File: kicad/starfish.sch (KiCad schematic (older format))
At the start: 3 parts, among them J1 Conn_02x04_Counter_Clockwise, J2 Conn_01x04, U1 kmz60

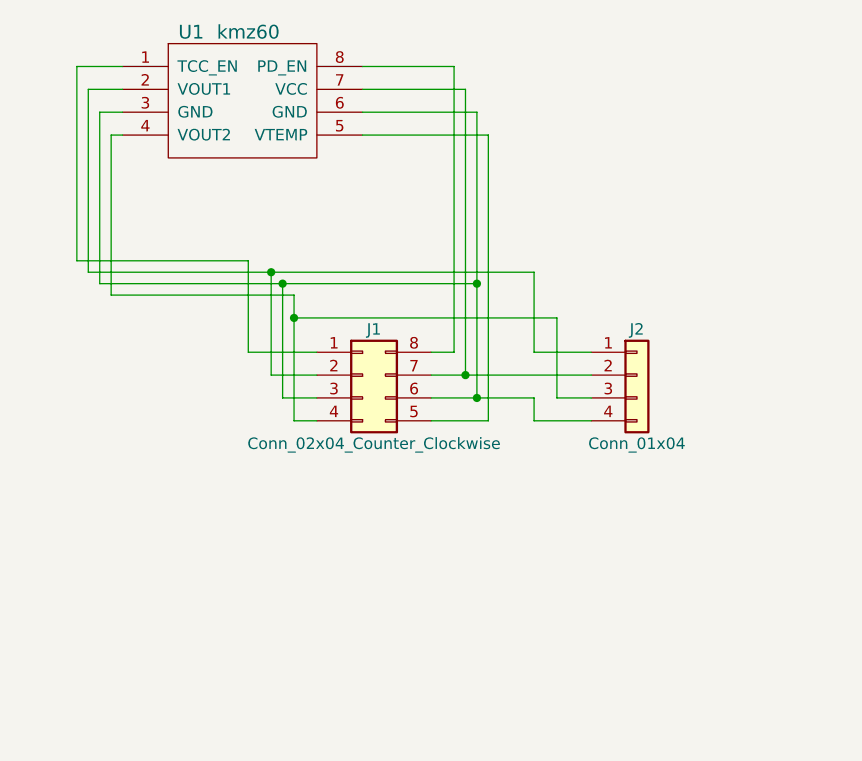
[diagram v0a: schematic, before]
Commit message: kicad
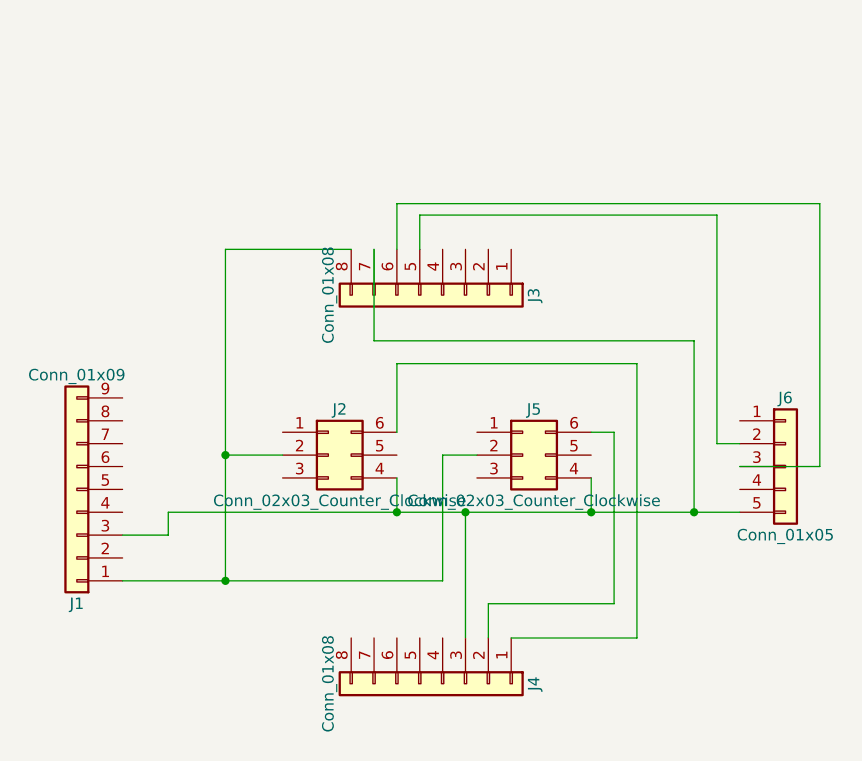
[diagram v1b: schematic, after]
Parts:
- removed J1: Conn_02x04_Counter_Clockwise, Pin_Headers:Pin_Header_Straight_2x04_Pitch2.54mm, symbol Conn_02x04_Counter_Clockwise
- removed J2: Conn_01x04, Pin_Headers:Pin_Header_Straight_1x04_Pitch2.54mm, symbol Conn_01x04
- removed U1: kmz60, Housings_SOIC:SO-8_5.3x6.2mm_Pitch1.27mm, symbol kmz60
- added J1: Conn_01x09, Pin_Headers:Pin_Header_Straight_1x09_Pitch2.54mm, symbol Conn_01x09
- added J2, J5: Conn_02x03_Counter_Clockwise, Pin_Headers:Pin_Header_Straight_2x03_Pitch2.54mm, symbol Conn_02x03_Counter_Clockwise
- added J3, J4: Conn_01x08, Pin_Headers:Pin_Header_Straight_1x08_Pitch2.54mm, symbol Conn_01x08
- added J6: Conn_01x05, Pin_Headers:Pin_Header_Straight_1x05_Pitch2.54mm, symbol Conn_01x05
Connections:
- new net: J2.6 (Pin_6), J4.1 (Pin_1)
- new net: J4.2 (Pin_2), J5.6 (Pin_6)
- new net: J1.3 (Pin_3), J2.4 (Pin_4), J3.7 (Pin_7), J4.3 (Pin_3), J5.4 (Pin_4), J6.5 (Pin_5)
- new net: J1.1 (Pin_1), J2.2 (Pin_2), J3.8 (Pin_8), J5.2 (Pin_2)
- new net: J3.5 (Pin_5), J6.2 (Pin_2)
- new net: J3.6 (Pin_6), J6.3 (Pin_3)
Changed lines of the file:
@@
 $EndDescr
 $Comp
-L kmz60 U1
-U 1 1 5ACC2B76
-P 5100 2750
-F 0 "U1" H 4900 3050 60  0000 C CNN
-F 1 "kmz60" H 5150 3050 60  0000 C CNN
-F 2 "Housings_SOIC:SO-8_5.3x6.2mm_Pitch1.27mm" H 5150 2750 60  0001 C CNN
-F 3 "" H 5150 2750 60  0001 C CNN
-	1    5100 2750
+L Conn_01x08 J4
+U 1 1 5ACD637F
+P 6000 5300
+F 0 "J4" H 6000 5700 50  0000 C CNN
+F 1 "Conn_01x08" H 6000 4800 50  0000 C CNN
+F 2 "Pin_Headers:Pin_Header_Straight_1x08_Pitch2.54mm" H 6000 5300 50  0001 C CNN
+F 3 "" H 6000 5300 50  0001 C CNN
+	1    6000 5300
+	0    1    1    0
+$EndComp
+$Comp
+L Conn_01x09 J1
+U 1 1 5ACD6458
+P 4400 4450
+F 0 "J1" H 4400 4950 50  0000 C CNN
+F 1 "Conn_01x09" H 4400 3950 50  0000 C CNN
+F 2 "Pin_Headers:Pin_Header_Straight_1x09_Pitch2.54mm" H 4400 4450 50  0001 C CNN
+F 3 "" H 4400 4450 50  0001 C CNN
+	1    4400 4450
+	-1   0    0    1
+$EndComp
+$Comp
+L Conn_01x05 J6
+U 1 1 5ACD64AB
+P 7500 4350
+F 0 "J6" H 7500 4650 50  0000 C CNN
+F 1 "Conn_01x05" H 7500 4050 50  0000 C CNN
+F 2 "Pin_Headers:Pin_Header_Straight_1x05_Pitch2.54mm" H 7500 4350 50  0001 C CNN
+F 3 "" H 7500 4350 50  0001 C CNN
+	1    7500 4350
 	1    0    0    -1
 $EndComp
 $Comp
-L Conn_01x04 J2
-U 1 1 5ACCDD93
-P 6850 3950
-F 0 "J2" H 6850 4150 50  0000 C CNN
-F 1 "Conn_01x04" H 6850 3650 50  0000 C CNN
-F 2 "Pin_Headers:Pin_Header_Straight_1x04_Pitch2.54mm" H 6850 3950 50  0001 C CNN
-F 3 "" H 6850 3950 50  0001 C CNN
-	1    6850 3950
+L Conn_01x08 J3
+U 1 1 5ACD6582
+P 6000 3600
+F 0 "J3" H 6000 4000 50  0000 C CNN
+F 1 "Conn_01x08" H 6000 3100 50  0000 C CNN
+F 2 "Pin_Headers:Pin_Header_Straight_1x08_Pitch2.54mm" H 6000 3600 50  0001 C CNN
+F 3 "" H 6000 3600 50  0001 C CNN
+	1    6000 3600
+	0    1    1    0
+$EndComp
+$Comp
+L Conn_02x03_Counter_Clockwise J2
+U 1 1 5ACD65C4
+P 5500 4300
+F 0 "J2" H 5550 4500 50  0000 C CNN
+F 1 "Conn_02x03_Counter_Clockwise" H 5550 4100 50  0000 C CNN
+F 2 "Pin_Headers:Pin_Header_Straight_2x03_Pitch2.54mm" H 5500 4300 50  0001 C CNN
+F 3 "" H 5500 4300 50  0001 C CNN
+	1    5500 4300
 	1    0    0    -1
 $EndComp
 $Comp
-L Conn_02x04_Counter_Clockwise J1
-U 1 1 5ACCDDC6
-P 5650 3950
-F 0 "J1" H 5700 4150 50  0000 C CNN
-F 1 "Conn_02x04_Counter_Clockwise" H 5700 3650 50  0000 C CNN
-F 2 "Pin_Headers:Pin_Header_Straight_2x04_Pitch2.54mm" H 5650 3950 50  0001 C CNN
-F 3 "" H 5650 3950 50  0001 C CNN
-	1    5650 3950
+L Conn_02x03_Counter_Clockwise J5
+U 1 1 5ACD664C
+P 6350 4300
+F 0 "J5" H 6400 4500 50  0000 C CNN
+F 1 "Conn_02x03_Counter_Clockwise" H 6400 4100 50  0000 C CNN
+F 2 "Pin_Headers:Pin_Header_Straight_2x03_Pitch2.54mm" H 6350 4300 50  0001 C CNN
+F 3 "" H 6350 4300 50  0001 C CNN
+	1    6350 4300
 	1    0    0    -1
 $EndComp
 Wire Wire Line
-	4600 2600 4400 2600
+	5300 4300 5050 4300
 Wire Wire Line
-	4400 2600 4400 3450
+	5050 3400 5050 4850
 Wire Wire Line
-	4400 3450 5150 3450
+	4600 4850 6000 4850
 Wire Wire Line
-	5150 3450 5150 3850
+	6000 4850 6000 4300
 Wire Wire Line
-	5150 3850 5450 3850
+	6000 4300 6150 4300
+Connection ~ 5050 4850
 Wire Wire Line
-	4600 2700 4450 2700
+	5050 3400 5600 3400
+Connection ~ 5050 4300
 Wire Wire Line
-	4450 2700 4450 3500
+	5800 4200 5800 3900
 Wire Wire Line
-	4450 3500 6400 3500
+	5800 3900 6850 3900
 Wire Wire Line
-	5250 3500 5250 3950
+	6850 3900 6850 5100
 Wire Wire Line
-	5250 3950 5450 3950
+	6850 5100 6300 5100
 Wire Wire Line
-	4600 2800 4500 2800
+	6650 4200 6750 4200
 Wire Wire Line
-	4500 2800 4500 3550
+	6750 4200 6750 4950
 Wire Wire Line
-	4500 3550 6150 3550
+	6750 4950 6200 4950
 Wire Wire Line
-	5300 3550 5300 4050
+	6200 4950 6200 5100
 Wire Wire Line
-	5300 4050 5450 4050
+	5800 3400 5800 3200
 Wire Wire Line
-	4600 2900 4550 2900
+	5800 3200 7650 3200
 Wire Wire Line
-	4550 2900 4550 3600
+	5900 3250 5900 3400
 Wire Wire Line
-	4550 3600 5350 3600
+	5700 3400 5700 3800
 Wire Wire Line
-	5350 3600 5350 4150
+	5700 3800 7100 3800
 Wire Wire Line
-	5350 4150 5450 4150
+	7100 3800 7100 4550
 Wire Wire Line
-	5650 2600 6050 2600
+	4800 4550 7300 4550
 Wire Wire Line
-	6050 2600 6050 3850
+	6100 4550 6100 5100
+Connection ~ 7100 4550
 Wire Wire Line
-	6050 3850 5950 3850
+	4800 4550 4800 4650
 Wire Wire Line
-	5650 2700 6100 2700
+	4800 4650 4600 4650
+Connection ~ 6100 4550
 Wire Wire Line
-	6100 2700 6100 3950
+	5800 4400 5800 4550
+Connection ~ 5800 4550
 Wire Wire Line
-	5950 3950 6650 3950
+	6650 4400 6650 4550
+Connection ~ 6650 4550
 Wire Wire Line
-	5650 2800 6150 2800
+	5900 3250 7200 3250
 Wire Wire Line
-	6150 2800 6150 4050
+	7200 3250 7200 4250
 Wire Wire Line
-	5950 4050 6400 4050
+	7200 4250 7300 4250
 Wire Wire Line
-	5650 2900 6200 2900
+	7650 3200 7650 4350
 Wire Wire Line
-	6200 2900 6200 4150
-Wire Wire Line
-	6200 4150 5950 4150
-Connection ~ 6100 3950
-Wire Wire Line
-	6400 4050 6400 4150
-Wire Wire Line
-	6400 4150 6650 4150
-Connection ~ 6150 4050
-Wire Wire Line
-	6400 3500 6400 3850
-Wire Wire Line
-	6400 3850 6650 3850
-Connection ~ 5250 3500
-Wire Wire Line
-	5350 3700 6500 3700
-Wire Wire Line
-	6500 3700 6500 4050
-Wire Wire Line
-	6500 4050 6650 4050
-Connection ~ 5350 3700
-Connection ~ 6150 3550
-Connection ~ 5300 3550
+	7650 4350 7300 4350
 $EndSCHEMATC
